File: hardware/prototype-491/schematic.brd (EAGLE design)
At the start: 116.8 x 110.2 mm, 27 parts, among them IC1 LM2576T, IC2 LM2576T, J1 OBD_CONN, J2 SUPPLY, Q1 220mA/50V/3.5Ω, Q2 220mA/50V/3.5Ω

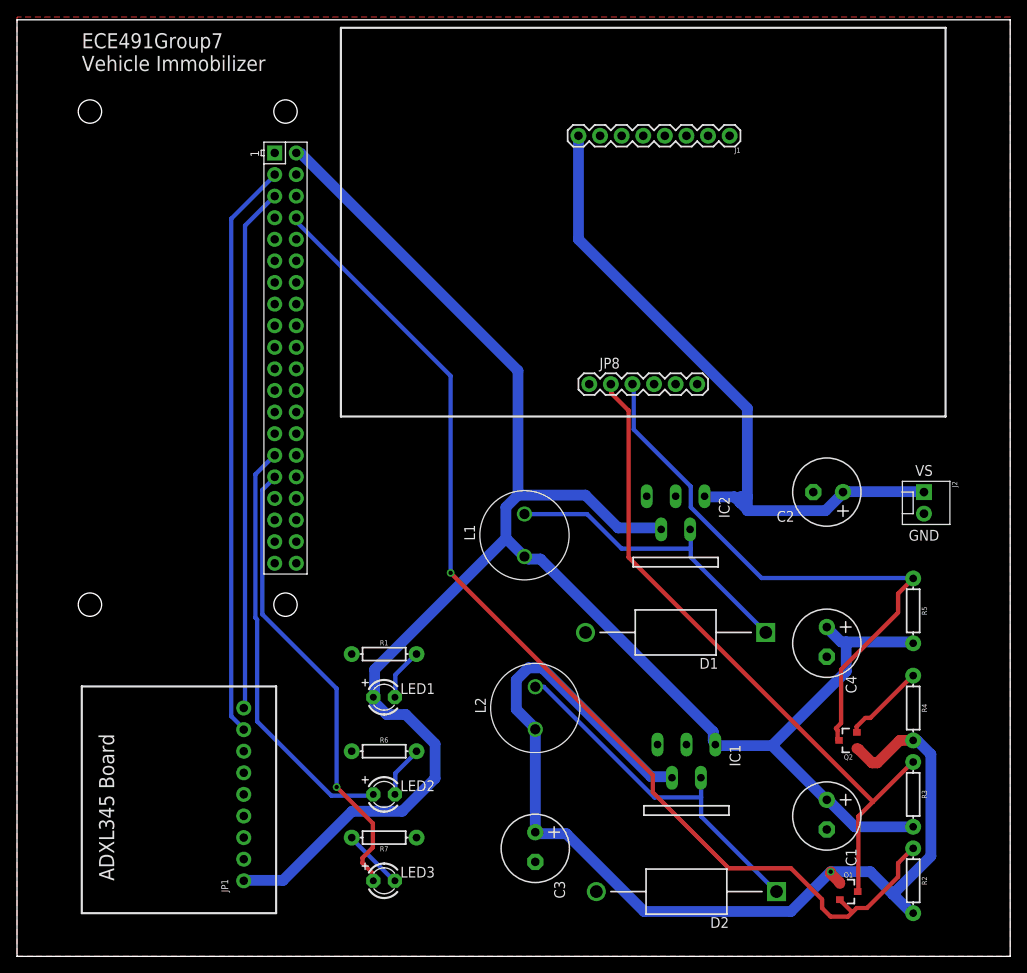
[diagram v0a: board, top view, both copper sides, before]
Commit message: test module updates
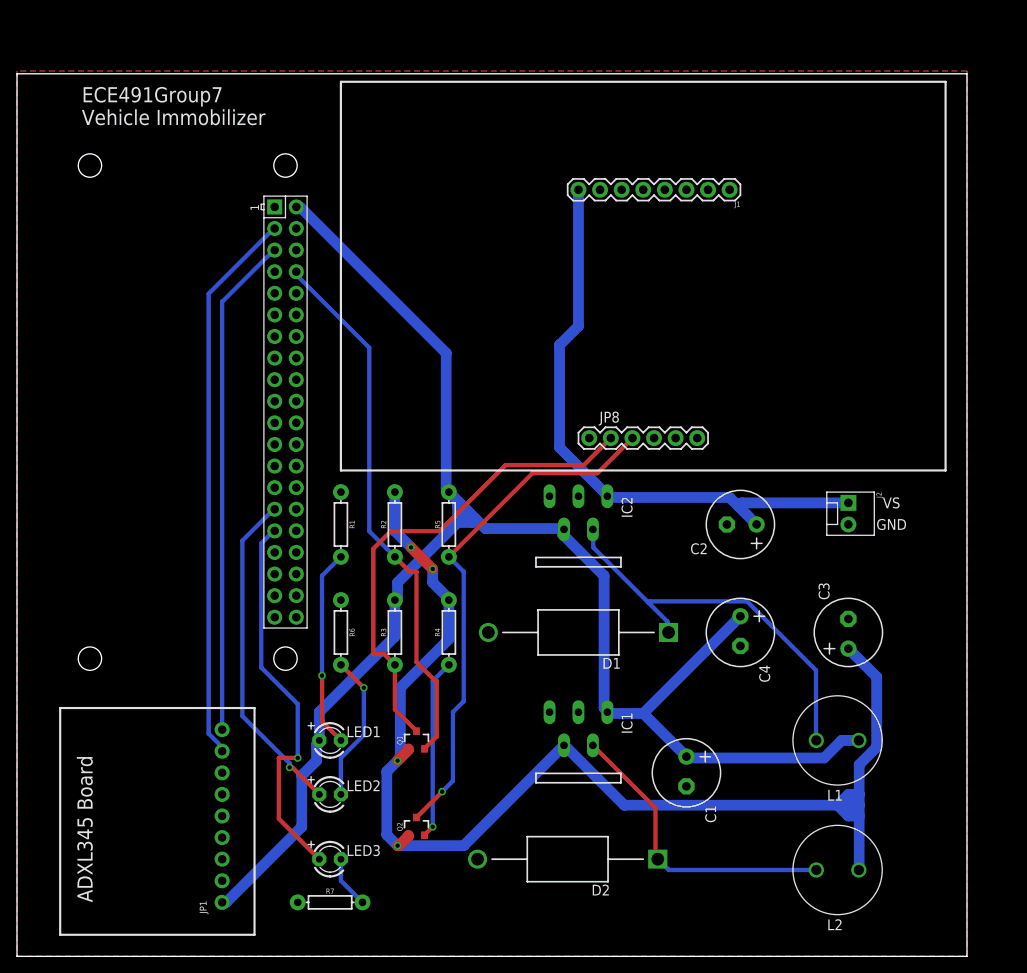
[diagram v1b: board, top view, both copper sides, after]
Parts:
- moved R2 74.0 mm to (44.5, 50.8), turned to 90 degrees
- moved R3 63.9 mm to (44.5, 38.1), turned to 90 degrees
- moved R5 55.5 mm to (50.8, 50.8), turned to 90 degrees
- moved R4 55.3 mm to (50.8, 38.1), turned to 90 degrees
- moved Q1 53.8 mm to (47.0, 25.4), turned to 0 degrees
- moved Q2 51.8 mm to (47.0, 15.2), turned to 0 degrees
- moved C3 44.7 mm to (97.8, 38.1), turned to 90 degrees
- moved L1 44.0 mm to (96.5, 25.4), turned to 0 degrees
- moved L2 40.3 mm to (96.5, 10.2), turned to 0 degrees
- moved C1 17.3 mm to (78.7, 21.6)
- moved R1 16.1 mm to (38.1, 50.8), turned to 270 degrees
- moved R6 14.9 mm to (38.1, 38.1), turned to 270 degrees
- moved D2 14.5 mm to (64.8, 11.4)
- moved IC1 13.3 mm to (66.0, 20.3)
- moved D1 11.4 mm to (66.0, 38.1)
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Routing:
- net TX_3V3: track 128.5 -> 64.1 mm, vias 1 -> 0
- net +5V: track 231.4 -> 192.0 mm
- net TX_5V: track 79.8 -> 57.6 mm
- net 3.3V: track 126.9 -> 148.0 mm, vias 1 -> 4
- net N$9: track 6.19 -> 23.4 mm, vias 0 -> 1
- net RX_3V3: track 9.81 -> 21.2 mm, vias 0 -> 1
- net N$5: track 6.12 -> 17.5 mm, vias 0 -> 1
- net N$2: track 49.7 -> 39.1 mm, vias 0 -> 1
- net N$4: track 37.1 -> 47.3 mm
- net VBAT: track 81.4 -> 71.3 mm
- net N$3: track 54.5 -> 45.3 mm
- net RX_5V: track 70.1 -> 61.1 mm, vias 0 -> 1
- net N$1: track 42.0 -> 35.9 mm
- net SCL: track 61.8 -> 59.0 mm
- net SDA: track 68.0 -> 65.4 mm
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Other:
- board size 116.8 x 110.2 mm -> 111.7 x 103.8 mm
